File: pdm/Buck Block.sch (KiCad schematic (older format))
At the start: 24 parts, among them Q10 2N7002E, Q11 2N7002E, Q15 Si7141DP, U7 BTS443P, U8 LM5085

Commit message: completed BoM
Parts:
- C12, C16, C18, C23: footprint Capacitor_SMD:C_0603_1608Metric -> Capacitor_SMD:C_0805_2012Metric; Digi-Key_PN (none) -> 445-14423-2-ND
- L1: footprint Inductor_SMD:L_Wuerth_HCM-1390 -> pdm_v2:inductor-PA4349.103ANLT; Digi-Key_PN (none) -> 553-4048-1-ND; MFR_PN 744309025 -> (none)
- Q15: Digi-Key_PN (none) -> SI7141DP-T1-GE3CT-ND
- U7: Digi-Key_PN (none) -> BTS443PAUMA1CT-ND
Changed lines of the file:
@@
 F 2 "Package_TO_SOT_SMD:TO-252-4" H 2800 2700 50  0001 C CNN
 F 3 "http://www.infineon.com/dgdl/Infineon-BTS443P-DS-v01_00-EN.pdf?fileId=5546d4625a888733015aa9afbc5035d5" H 2800 2550 50  0001 C CNN
+F 4 "BTS443PAUMA1CT-ND" H 2800 2950 50  0001 C CNN "Digi-Key_PN"
 	1    2800 2950
 	1    0    0    -1
@@
 F 0 "C18" H 3635 3354 50  0000 R CNN
 F 1 "15uF" H 3635 3445 50  0000 R CNN
-F 2 "Capacitor_SMD:C_0603_1608Metric" H 3788 3250 50  0001 C CNN
+F 2 "Capacitor_SMD:C_0805_2012Metric" H 3788 3250 50  0001 C CNN
 F 3 "~" H 3750 3400 50  0001 C CNN
+F 4 "445-14423-2-ND" H 3750 3400 50  0001 C CNN "Digi-Key_PN"
 	1    3750 3400
 	-1   0    0    1
@@
 F 0 "L1" V 9640 2950 50  0000 C CNN
 F 1 "3.3uH" V 9549 2950 50  0000 C CNN
-F 2 "Inductor_SMD:L_Wuerth_HCM-1390" H 9450 2950 50  0001 C CNN
-F 3 "~" H 9450 2950 50  0001 C CNN
-F 4 "744309025" H 9450 2950 50  0001 C CNN "MFR_PN"
+F 2 "pdm_v2:inductor-PA4349.103ANLT" H 9450 2950 50  0001 C CNN
+F 3 "https://media.digikey.com/pdf/Data%20Sheets/Pulse%20PDFs/PA4349.zzzANLT_Series_Rev2019.pdf" H 9450 2950 50  0001 C CNN
+F 4 "" H 9450 2950 50  0001 C CNN "MFR_PN"
+F 5 "553-4048-1-ND" H 9450 2950 50  0001 C CNN "Digi-Key_PN"
 	1    9450 2950
 	0    -1   -1   0
@@
 F 0 "C23" H 10465 3496 50  0000 L CNN
 F 1 "15uF" H 10465 3405 50  0000 L CNN
-F 2 "Capacitor_SMD:C_0603_1608Metric" H 10388 3300 50  0001 C CNN
+F 2 "Capacitor_SMD:C_0805_2012Metric" H 10388 3300 50  0001 C CNN
 F 3 "~" H 10350 3450 50  0001 C CNN
+F 4 "445-14423-2-ND" H 10350 3450 50  0001 C CNN "Digi-Key_PN"
 	1    10350 3450
 	1    0    0    -1
@@
 F 0 "C12" H 4085 3354 50  0000 R CNN
 F 1 "15uF" H 4085 3445 50  0000 R CNN
-F 2 "Capacitor_SMD:C_0603_1608Metric" H 4238 3250 50  0001 C CNN
+F 2 "Capacitor_SMD:C_0805_2012Metric" H 4238 3250 50  0001 C CNN
 F 3 "~" H 4200 3400 50  0001 C CNN
+F 4 "445-14423-2-ND" H 4200 3400 50  0001 C CNN "Digi-Key_PN"
 	1    4200 3400
 	-1   0    0    1
@@
 F 0 "C16" H 4535 3354 50  0000 R CNN
 F 1 "15uF" H 4535 3445 50  0000 R CNN
-F 2 "Capacitor_SMD:C_0603_1608Metric" H 4688 3250 50  0001 C CNN
+F 2 "Capacitor_SMD:C_0805_2012Metric" H 4688 3250 50  0001 C CNN
 F 3 "~" H 4650 3400 50  0001 C CNN
+F 4 "445-14423-2-ND" H 4650 3400 50  0001 C CNN "Digi-Key_PN"
 	1    4650 3400
 	-1   0    0    1
@@
 F 2 "Package_SO:PowerPAK_SO-8_Single" H 8800 2975 50  0001 L CIN
 F 3 "https://www.vishay.com/docs/65596/si7141dp.pdf" H 8600 3050 50  0001 L CNN
+F 4 "SI7141DP-T1-GE3CT-ND" H 8600 3050 50  0001 C CNN "Digi-Key_PN"
 	1    8600 3050
 	0    -1   -1   0

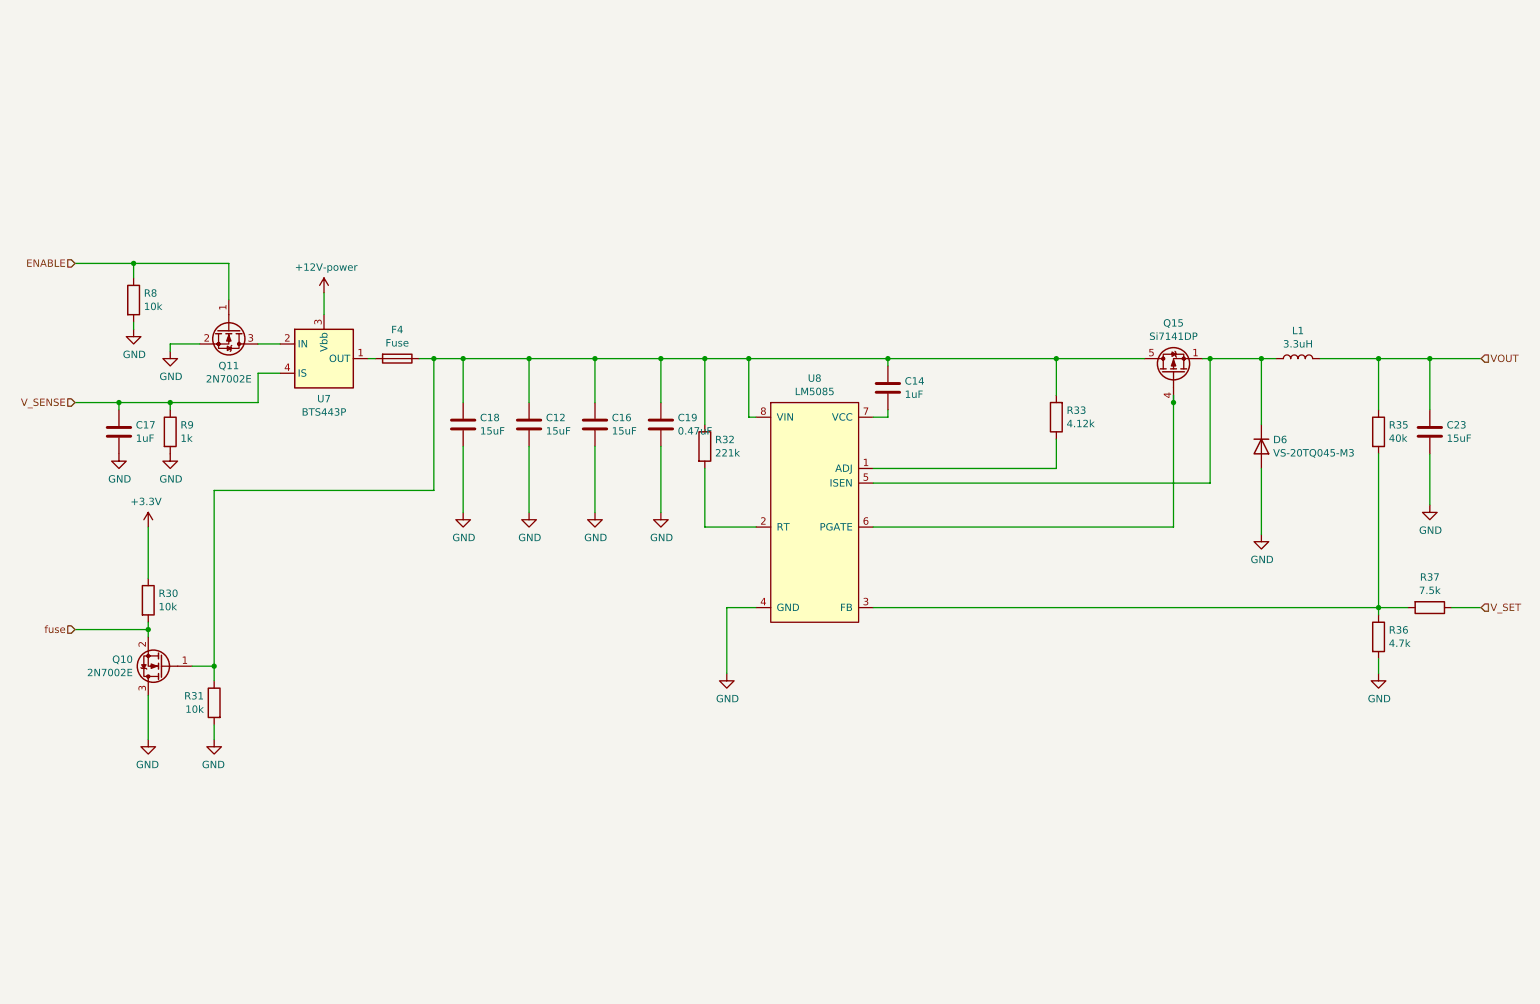
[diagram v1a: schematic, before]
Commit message: general changes
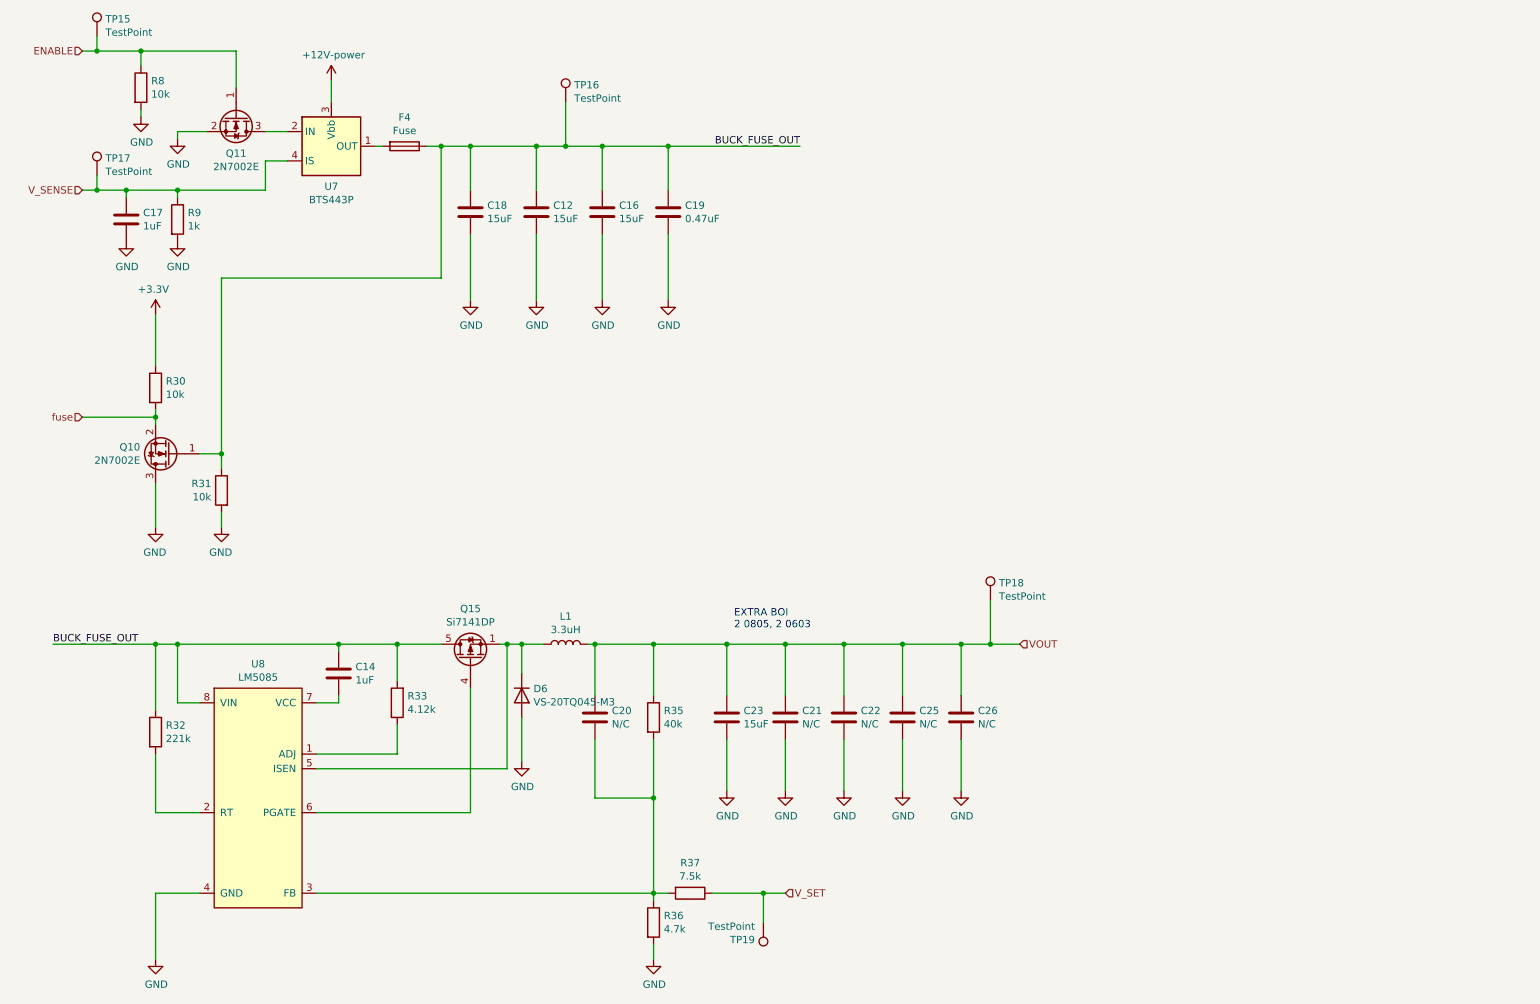
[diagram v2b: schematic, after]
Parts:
- added C20, C21, C22, C25, C26: N/C, Capacitor_SMD:C_0805_2012Metric, symbol Device:C
- added TP15, TP16, TP17, TP18, TP19: TestPoint, TestPoint:TestPoint_THTPad_1.0x1.0mm_Drill0.5mm, symbol Connector:TestPoint
- D6: footprint Package_TO_SOT_THT:TO-220-2_Vertical -> Package_TO_SOT_THT:TO-220-2_Horizontal_TabDown
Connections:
- net ENABLE: now also TP15.1
- net GND: now also C21.2, C22.2, C25.2, C26.2
- net VOUT: now also C20.1, C21.1, C22.1, C25.1, C26.1, TP18.1
- net V_SENSE: now also TP17.1
- net V_SET: now also TP19.1
- net at R35.2, R36.1, R37.2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: now also C20.2
- net BUCK_FUSE_OUT: now reaches C12.2, C14.2, C16.2, C18.2, C19.2, F4.1, Q10.1 (G), Q15.5 (D), R31.1, R32.1, R33.2, U8.8 (VIN)
- net BUCK_FUSE_OUT: now also TP16.1
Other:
- note added: "EXTRA BOI\n2 0805, 2 0603"
- moved on the sheet: C12, C14, C16, C17, C18, C19, C23, D6, F4, L1, Q10, Q11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
